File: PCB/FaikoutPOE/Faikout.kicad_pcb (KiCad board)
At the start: 2 copper layers, 42 x 69 mm, 87 parts, among them J1 RJ45_LED, J3 S21, J5 Reset, J7 TC2030-USB-NL-DS, M1 Ag9912-LP, P1 Square, P2 Square, P3 Square, P4 Square, Q1 BSS138PS, Q2 BSS138PS, U1 KSZ8851SNL, U2 ESP32-S3-MINI-1, U3 TCMT1100, U4 TPS62933, U5 TCMT1100, Y1 Crystal_GND24

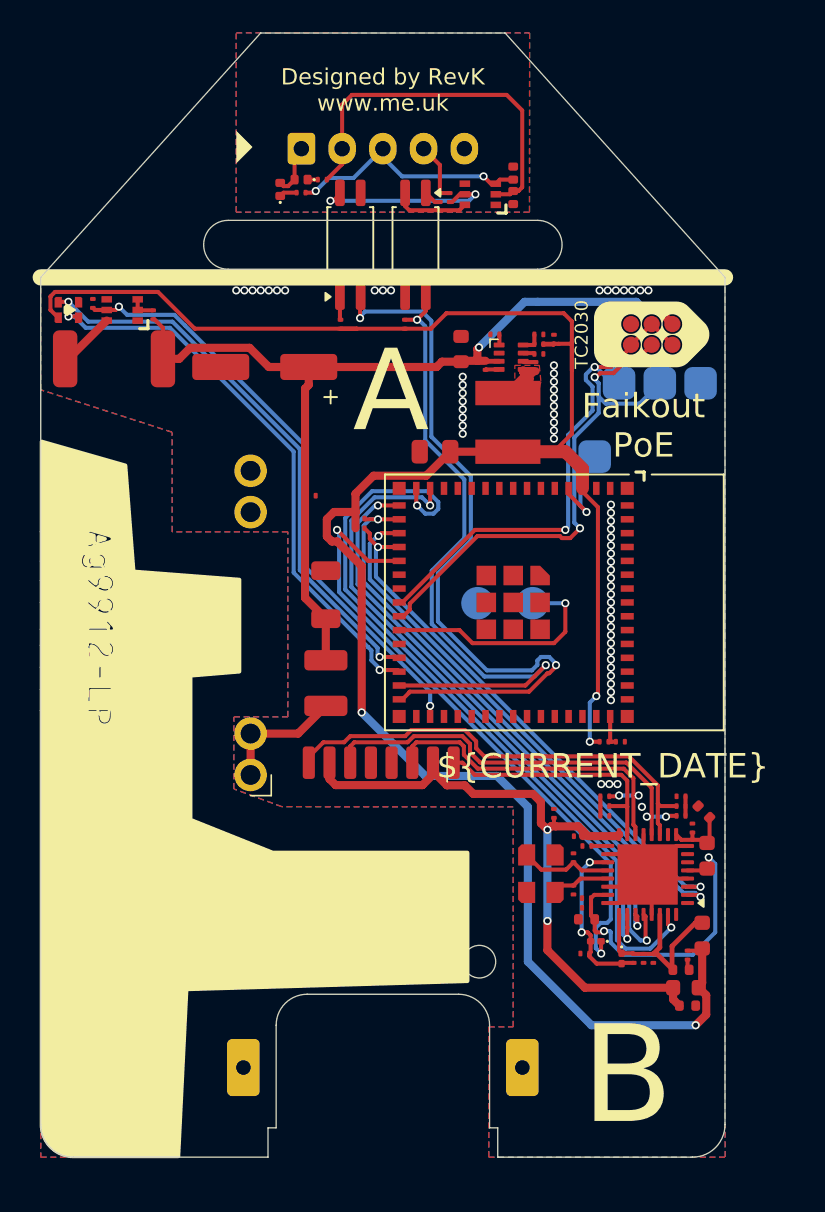
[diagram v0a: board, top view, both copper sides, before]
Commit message: Smaller design
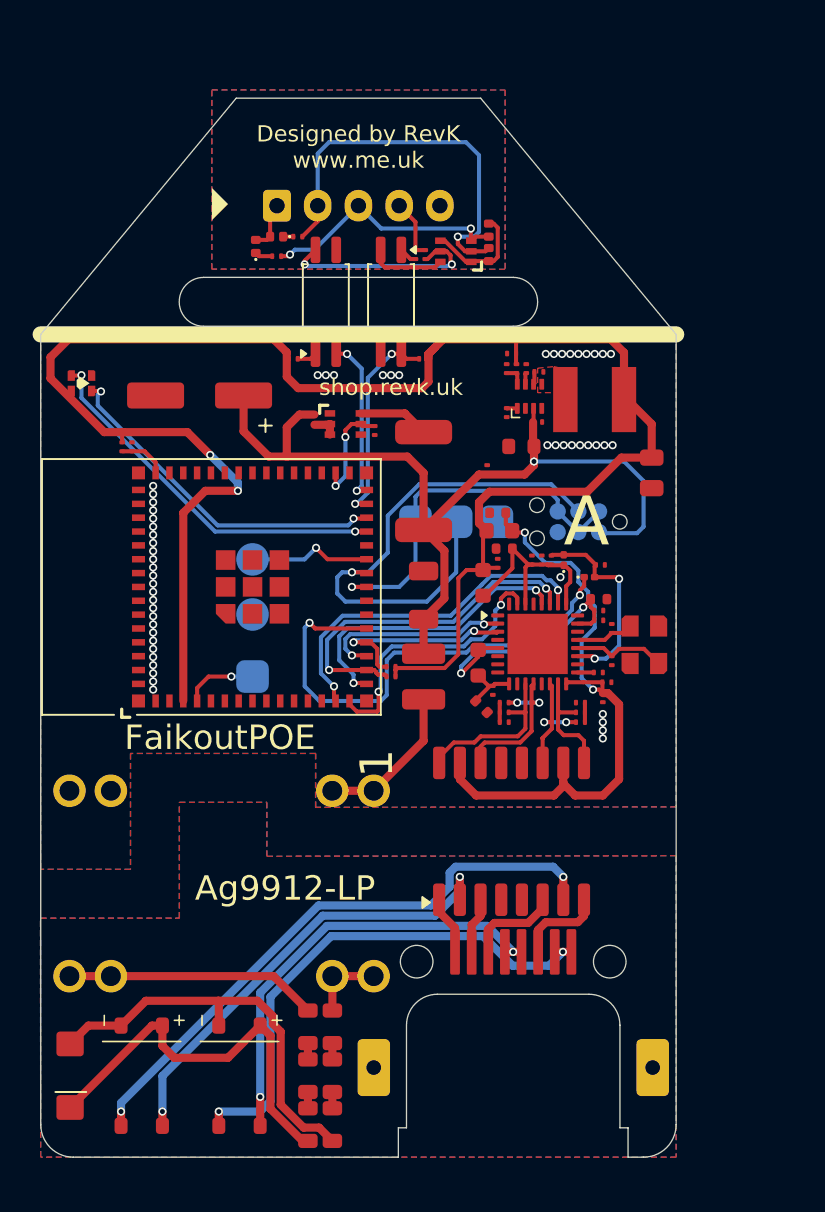
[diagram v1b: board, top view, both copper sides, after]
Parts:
- J7: moved to B.Cu
- moved C36 35.0 mm to (105.6, 56.4), turned to 90 degrees
- moved R9 34.7 mm to (105.0, 56.4), turned to -90 degrees
- moved C2 32.4 mm to (128.1, 60.5), turned to 180 degrees
- moved FB4 30.3 mm to (128.2, 61.5), turned to 180 degrees
- moved C5 28.0 mm to (128.4, 62.6), turned to 180 degrees
- moved C34 26.7 mm to (128.1, 63.5), turned to -90 degrees
- moved C3 25.6 mm to (130.2, 63.4), turned to 90 degrees
- moved FB5 25.5 mm to (127.2, 64.8), turned to 90 degrees
- moved C4 25.2 mm to (130.8, 63.4), turned to 90 degrees
- moved R7 25.0 mm to (131.3, 63.4), turned to 90 degrees
- moved P1 25.0 mm to (113.0, 70.5)
- moved D2 24.7 mm to (132.1, 63.4), turned to 90 degrees
- moved C16 23.9 mm to (134.3, 63.6), turned to 0 degrees
- moved D1 22.4 mm to (133.7, 64.4), turned to 0 degrees
- moved L14 20.9 mm to (116.4, 98.0), turned to 90 degrees
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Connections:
- J1 pad S1: unconnected-(J1-PadS1) -> VIN-
- J1 pad S2: GND -> VIN-
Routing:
- net TX: track 46.3 -> 10.2 mm
- net +3.3V: track 141.5 -> 110.5 mm, vias 4 -> 2
- net SI: track 47.6 -> 16.8 mm
- net POELOAD: track 36.5 -> 6.48 mm
- net RX: track 41.3 -> 12.7 mm
- net PME: track 33.5 -> 11.9 mm
- net GND: track 20.9 -> 0.00 mm, vias 64 -> 55
- net INTR: track 33.3 -> 12.5 mm
- net SCLK: track 37.9 -> 18.4 mm
- net CSN: track 40.9 -> 21.7 mm
- net RXP: track 28.4 -> 10.1 mm
- net RXN: track 26.4 -> 9.83 mm
- net E12: track 12.7 -> 28.3 mm, vias 0 -> 2
- net TXP: track 21.5 -> 7.57 mm
- net VIN+: track 29.4 -> 15.5 mm
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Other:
- board size 42 x 69 mm -> 39 x 65 mm
- board text added: "10/100 Ethernet PoE"
- board text added: "ABE"
- board text added: "FaikoutPOE"
- board text removed: "${CURRENT_DATE}"
- board text removed: "10/100 Ethernet"
- board text removed: "AB"
- board text removed: "B"
- board text removed: "E"
- board text removed: "Faikout PoE"
